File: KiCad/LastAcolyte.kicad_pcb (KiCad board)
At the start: 2 copper layers, 170 x 170 mm, 711 parts, among them J1 USB_B, J2 Mini-DIN-6, J3 AudioJack3, J4 DB15_Female_HighDensity, J5 Conn-01x06, J6 Conn_01x02, J7 Conn_02x20_Odd_Even, Q1 PN2222A, Q2 PN2222A, Q3 PN2222A, SW1 SW_SPDT, SW2 SW_Push, U1 W65C02SxP, U10 74HC273, U11 74HC166, U12 74HC166, U13 74HC10, U14 74HC08, U15 74HC00, U16 74HC02, U17 MCP130-xxxDxTO, U18 25LCxxx, U2 AS6C4008-55PCN, U3 SST39SF040, U4 74HC161, U5 74HC590, U6 74HC590, U7 74HC590, U8 74HC245, U9 74HC377, X1 CXO_DIP8/14

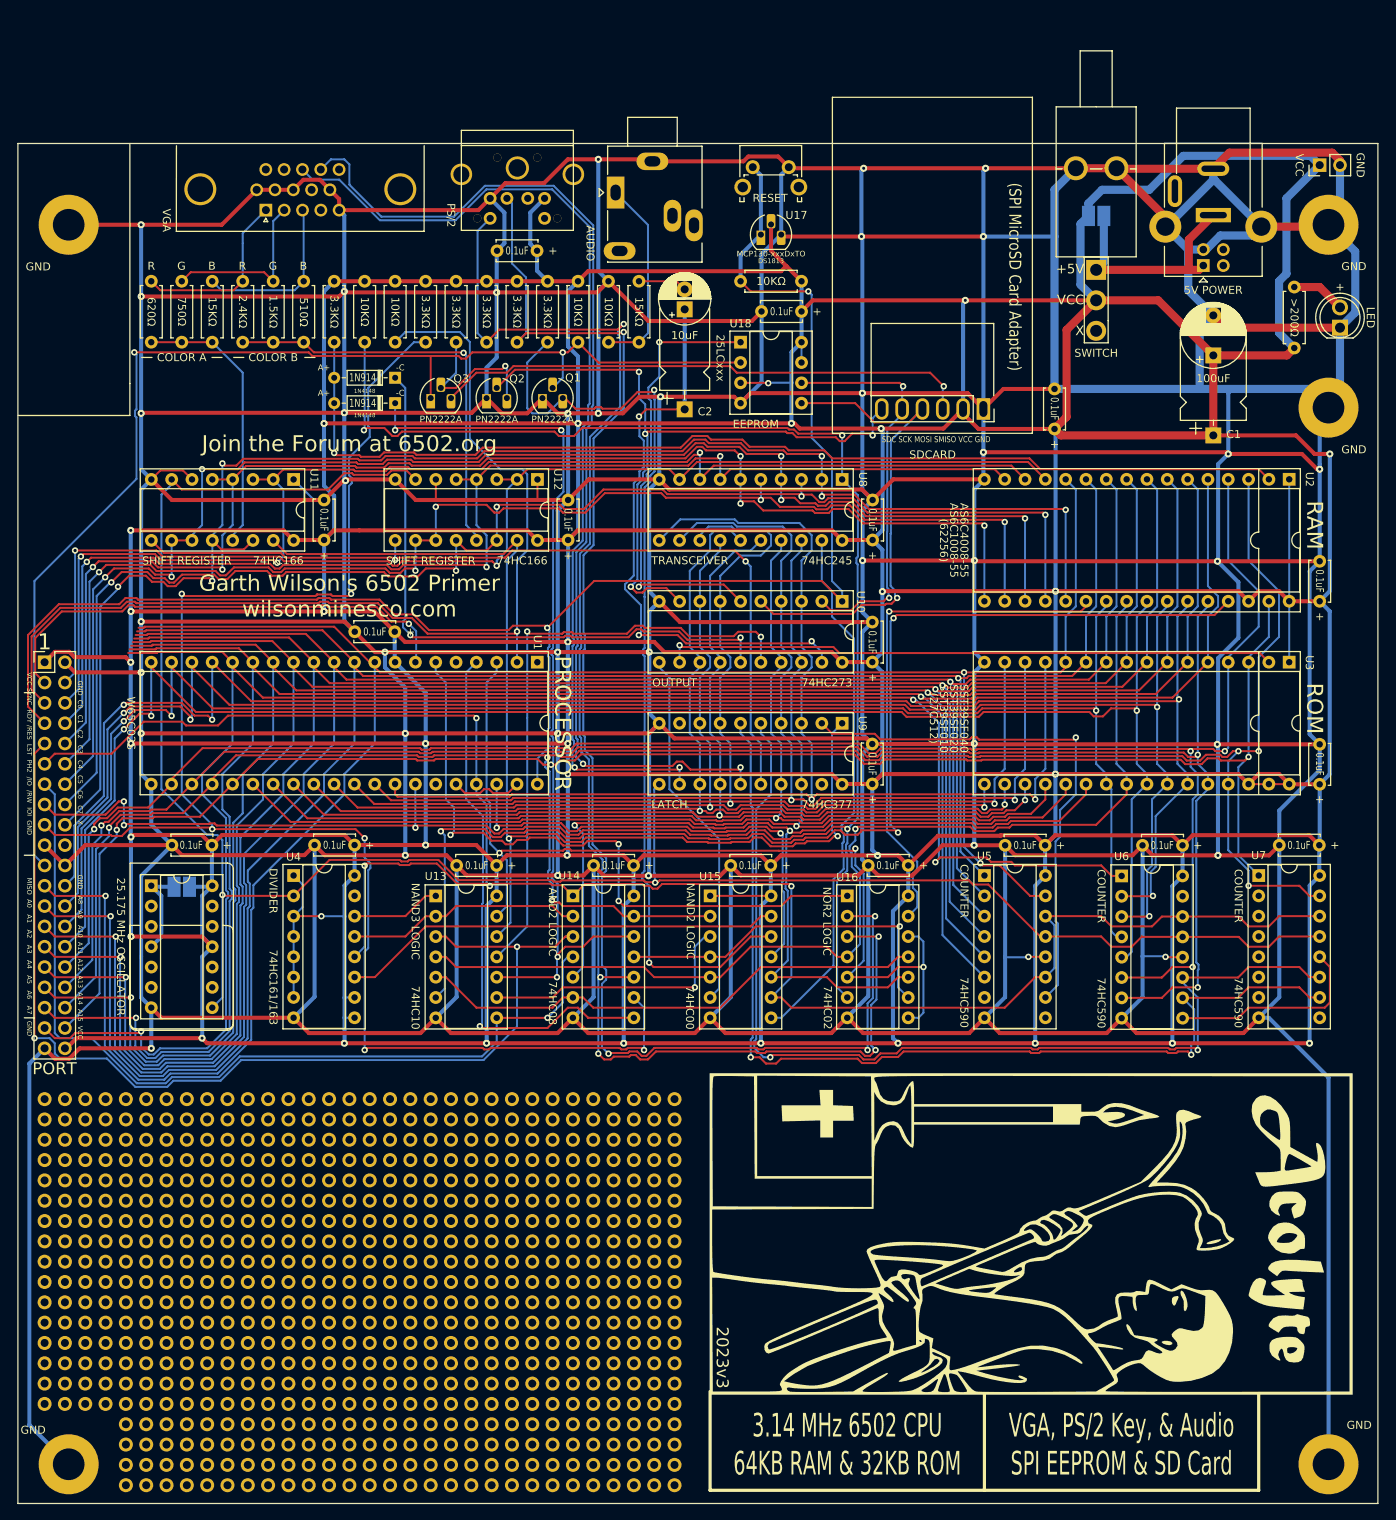
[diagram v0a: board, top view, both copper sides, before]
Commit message: Add files via upload
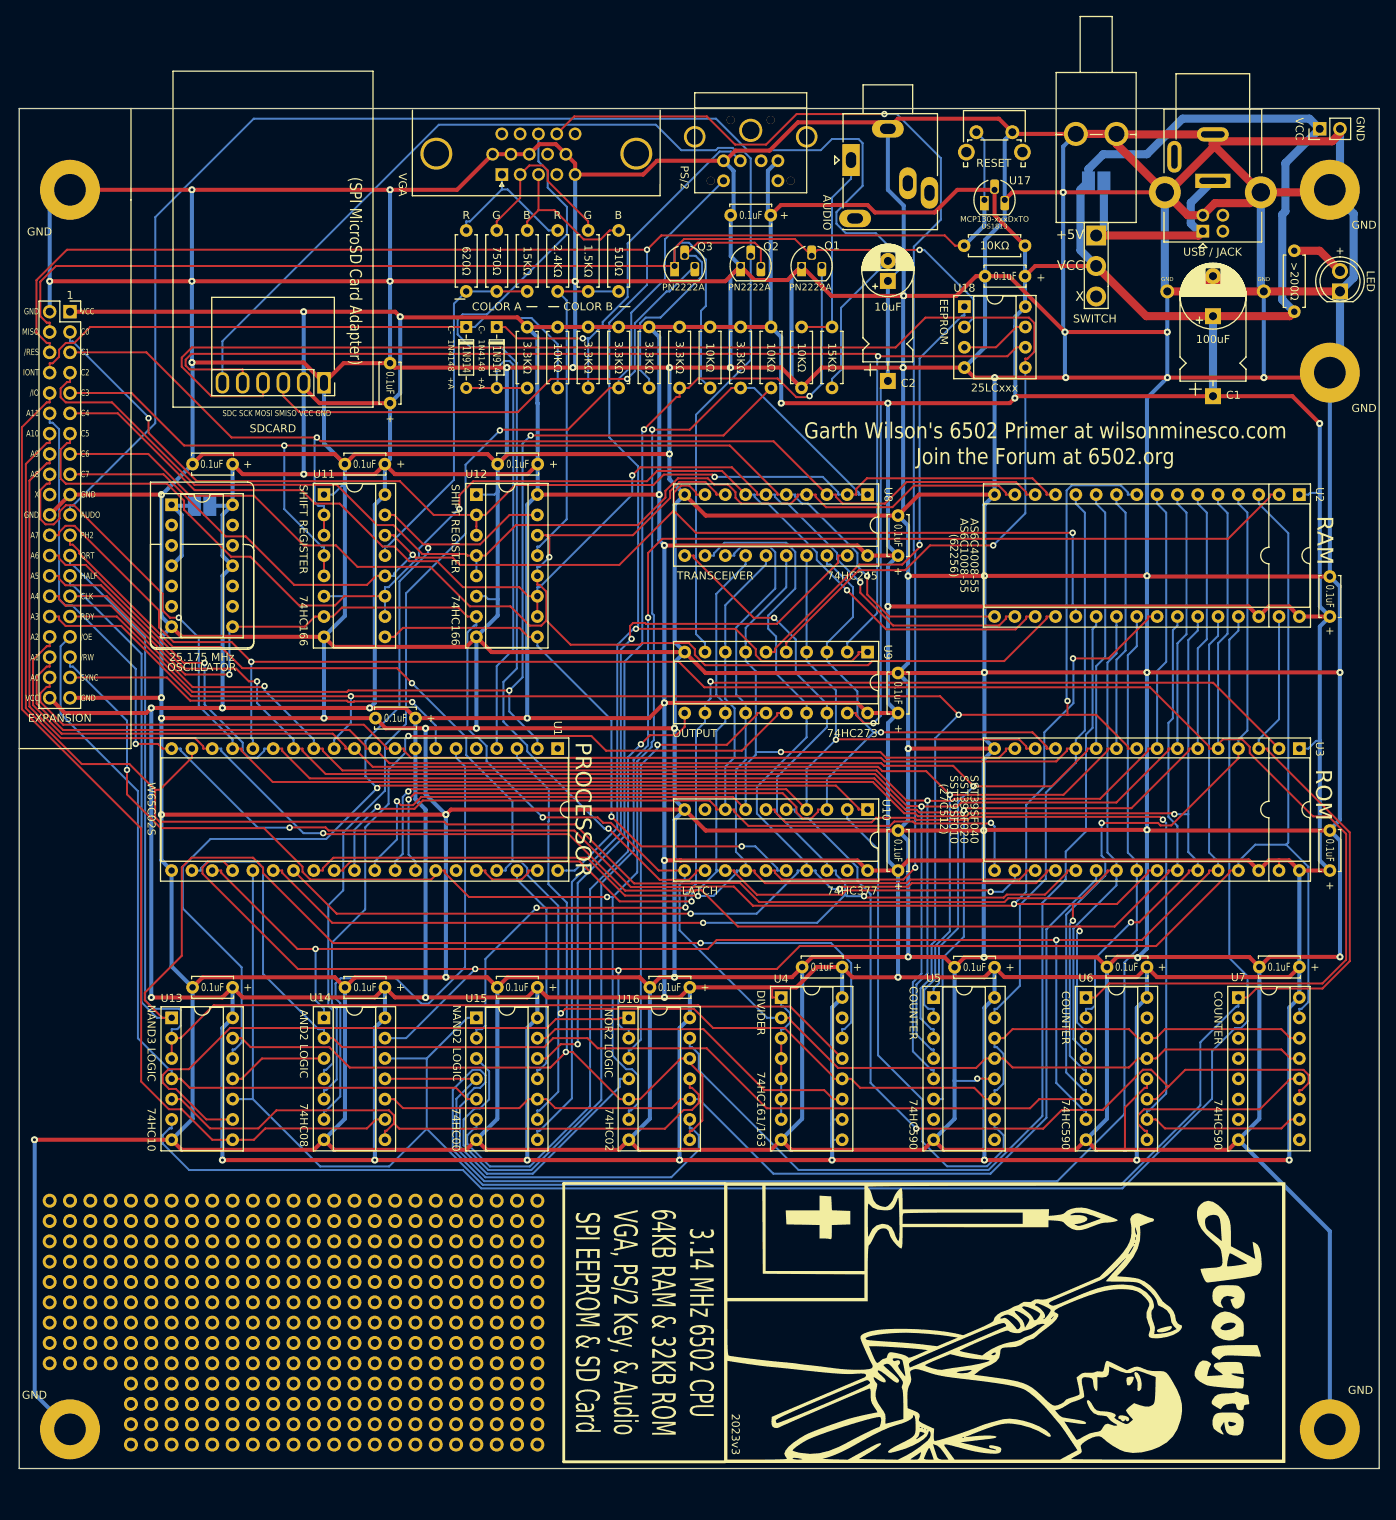
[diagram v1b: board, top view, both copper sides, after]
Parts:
- removed G100: LOGO, Library:Acolyte
- removed G200: LOGO, Library:GirlBW
- removed R15: R_US, Resistor_THT:R_Axial_DIN0207_L6.3mm_D2.5mm_P7.62mm_Horizontal
- removed the REF** at (40.0, 183.5)
- removed the REF** at (75.6, 155.6)
- removed the REF** at (101.0, 186.1)
- removed the REF** at (55.2, 181.0)
- removed the REF** at (40.0, 170.8)
- removed the REF** at (80.6, 160.7)
- removed the REF** at (29.8, 155.6)
- removed the REF** at (24.8, 170.8)
- removed the REF** at (34.9, 186.1)
- removed the REF** at (60.3, 178.4)
- removed the REF** at (98.4, 170.8)
- removed the REF** at (98.4, 145.4)
- removed the REF** at (85.7, 153.0)
- removed the REF** at (88.3, 186.1)
- removed the REF** at (50.2, 181.0)
- removed the REF** at (90.8, 188.6)
- removed the REF** at (83.2, 175.9)
- removed the REF** at (60.3, 183.5)
- removed the REF** at (75.6, 148.0)
- removed the REF** at (40.0, 173.4)
- removed the REF** at (101.0, 178.4)
- removed the REF** at (70.5, 165.7)
- removed the REF** at (60.3, 160.7)
- removed the REF** at (62.9, 165.7)
- removed the REF** at (85.7, 175.9)
- removed the REF** at (95.9, 170.8)
- removed the REF** at (27.3, 181.0)
- removed the REF** at (55.2, 165.7)
- removed the REF** at (75.6, 145.4)
- removed the REF** at (67.9, 160.7)
- removed the REF** at (50.2, 145.4)
- removed the REF** at (32.4, 186.1)
- removed the REF** at (101.0, 183.5)
- removed the REF** at (29.8, 170.8)
- removed the REF** at (95.9, 186.1)
- removed the REF** at (47.6, 158.1)
- removed the REF** at (52.7, 153.0)
- removed the REF** at (50.2, 163.2)
- removed the REF** at (67.9, 178.4)
- removed the REF** at (70.5, 150.5)
- removed the REF** at (57.8, 181.0)
- removed the REF** at (34.9, 145.4)
- removed the REF** at (29.8, 178.4)
- removed the REF** at (40.0, 160.7)
- removed the REF** at (101.0, 160.7)
- removed the REF** at (34.9, 173.4)
- removed the REF** at (42.5, 191.1)
- removed the REF** at (50.2, 193.7)
- removed the REF** at (65.4, 150.5)
- removed the REF** at (22.2, 150.5)
- removed the REF** at (73.0, 191.1)
- removed the REF** at (45.1, 188.6)
- removed the REF** at (101.0, 163.2)
- removed the REF** at (34.9, 160.7)
- removed the REF** at (60.3, 188.6)
- removed the REF** at (42.5, 165.7)
- removed the REF** at (22.2, 170.8)
- removed the REF** at (67.9, 150.5)
- removed the REF** at (27.3, 155.6)
- removed the REF** at (98.4, 193.7)
- removed the REF** at (62.9, 153.0)
- removed the REF** at (57.8, 186.1)
- removed the REF** at (80.6, 153.0)
- removed the REF** at (24.8, 175.9)
- removed the REF** at (70.5, 145.4)
- removed the REF** at (90.8, 160.7)
- removed the REF** at (73.0, 148.0)
- removed the REF** at (85.7, 155.6)
- removed the REF** at (57.8, 160.7)
- removed the REF** at (55.2, 186.1)
- removed the REF** at (52.7, 170.8)
- removed the REF** at (45.1, 155.6)
- removed the REF** at (57.8, 188.6)
- removed the REF** at (95.9, 148.0)
- removed the REF** at (32.4, 148.0)
- removed the REF** at (22.2, 183.5)
- removed the REF** at (65.4, 165.7)
- removed the REF** at (52.7, 150.5)
- removed the REF** at (34.9, 163.2)
- removed the REF** at (75.6, 178.4)
- removed the REF** at (50.2, 188.6)
- removed the REF** at (27.3, 173.4)
- removed the REF** at (101.0, 155.6)
- removed the REF** at (78.1, 168.3)
- removed the REF** at (95.9, 175.9)
- removed the REF** at (29.8, 173.4)
- removed the REF** at (45.1, 193.7)
- removed the REF** at (78.1, 183.5)
- removed the REF** at (27.3, 153.0)
- removed the REF** at (93.3, 160.7)
- removed the REF** at (70.5, 158.1)
- removed the REF** at (47.6, 155.6)
- removed the REF** at (73.0, 175.9)
- removed the REF** at (98.4, 173.4)
- removed the REF** at (37.5, 170.8)
- removed the REF** at (88.3, 193.7)
- removed the REF** at (62.9, 181.0)
- removed the REF** at (65.4, 163.2)
- removed the REF** at (75.6, 165.7)
- removed the REF** at (98.4, 175.9)
- removed the REF** at (50.2, 158.1)
- removed the REF** at (83.2, 188.6)
- removed the REF** at (88.3, 158.1)
- removed the REF** at (65.4, 148.0)
- removed the REF** at (85.7, 150.5)
- removed the REF** at (29.8, 150.5)
- removed the REF** at (47.6, 175.9)
- removed the REF** at (34.9, 175.9)
- removed the REF** at (85.7, 168.3)
- removed the REF** at (57.8, 170.8)
- removed the REF** at (47.6, 165.7)
- removed the REF** at (62.9, 148.0)
- removed the REF** at (42.5, 145.4)
- removed the REF** at (45.1, 191.1)
- removed the REF** at (75.6, 163.2)
- removed the REF** at (95.9, 145.4)
- removed the REF** at (32.4, 155.6)
- removed the REF** at (47.6, 168.3)
- removed the REF** at (65.4, 153.0)
- removed the REF** at (32.4, 150.5)
- removed the REF** at (60.3, 150.5)
- removed the REF** at (47.6, 148.0)
- removed the REF** at (88.3, 165.7)
- removed the REF** at (70.5, 181.0)
- removed the REF** at (42.5, 186.1)
- removed the REF** at (73.0, 173.4)
- removed the REF** at (67.9, 191.1)
- removed the REF** at (78.1, 163.2)
- removed the REF** at (57.8, 175.9)
- removed the REF** at (65.4, 191.1)
- removed the REF** at (27.3, 158.1)
- removed the REF** at (34.9, 170.8)
- removed the REF** at (55.2, 158.1)
- removed the REF** at (90.8, 181.0)
- removed the REF** at (78.1, 170.8)
- removed the REF** at (90.8, 153.0)
- removed the REF** at (83.2, 160.7)
- removed the REF** at (93.3, 150.5)
- removed the REF** at (80.6, 165.7)
- removed the REF** at (47.6, 183.5)
- removed the REF** at (73.0, 178.4)
- removed the REF** at (85.7, 191.1)
- removed the REF** at (88.3, 175.9)
- removed the REF** at (67.9, 183.5)
- removed the REF** at (60.3, 155.6)
- removed the REF** at (57.8, 178.4)
- removed the REF** at (50.2, 160.7)
- removed the REF** at (67.9, 170.8)
- removed the REF** at (85.7, 188.6)
- removed the REF** at (37.5, 186.1)
- removed the REF** at (55.2, 153.0)
- removed the REF** at (37.5, 178.4)
- removed the REF** at (78.1, 153.0)
- removed the REF** at (24.8, 155.6)
- removed the REF** at (50.2, 170.8)
- removed the REF** at (22.2, 155.6)
- removed the REF** at (90.8, 165.7)
- removed the REF** at (65.4, 173.4)
- removed the REF** at (93.3, 188.6)
- removed the REF** at (32.4, 165.7)
- removed the REF** at (83.2, 148.0)
- removed the REF** at (37.5, 153.0)
- removed the REF** at (95.9, 178.4)
- removed the REF** at (93.3, 191.1)
- removed the REF** at (90.8, 175.9)
- removed the REF** at (75.6, 186.1)
- removed the REF** at (55.2, 170.8)
- removed the REF** at (32.4, 173.4)
- removed the REF** at (42.5, 158.1)
- removed the REF** at (83.2, 193.7)
- removed the REF** at (83.2, 158.1)
- removed the REF** at (55.2, 145.4)
- removed the REF** at (34.9, 155.6)
- removed the REF** at (32.4, 160.7)
- removed the REF** at (24.8, 145.4)
- removed the REF** at (101.0, 153.0)
- removed the REF** at (83.2, 186.1)
- removed the REF** at (32.4, 158.1)
- removed the REF** at (93.3, 155.6)
- removed the REF** at (83.2, 170.8)
- removed the REF** at (90.8, 193.7)
- removed the REF** at (88.3, 148.0)
- removed the REF** at (22.2, 153.0)
- removed the REF** at (45.1, 168.3)
- removed the REF** at (95.9, 168.3)
- removed the REF** at (83.2, 145.4)
- removed the REF** at (95.9, 153.0)
- removed the REF** at (98.4, 178.4)
- removed the REF** at (93.3, 145.4)
- removed the REF** at (78.1, 193.7)
- removed the REF** at (40.0, 188.6)
- removed the REF** at (45.1, 148.0)
- removed the REF** at (47.6, 181.0)
- removed the REF** at (78.1, 148.0)
- removed the REF** at (50.2, 155.6)
- removed the REF** at (50.2, 178.4)
- removed the REF** at (101.0, 173.4)
- removed the REF** at (60.3, 153.0)
- removed the REF** at (62.9, 168.3)
- removed the REF** at (85.7, 148.0)
- removed the REF** at (60.3, 165.7)
- removed the REF** at (40.0, 150.5)
- removed the REF** at (50.2, 186.1)
- removed the REF** at (85.7, 165.7)
- removed the REF** at (27.3, 183.5)
- removed the REF** at (85.7, 186.1)
- removed the REF** at (37.5, 155.6)
- removed the REF** at (32.4, 145.4)
- removed the REF** at (65.4, 168.3)
- removed the REF** at (47.6, 163.2)
- removed the REF** at (80.6, 178.4)
- removed the REF** at (93.3, 153.0)
- removed the REF** at (93.3, 193.7)
- removed the REF** at (52.7, 191.1)
- removed the REF** at (73.0, 165.7)
- removed the REF** at (93.3, 173.4)
- removed the REF** at (70.5, 153.0)
- removed the REF** at (50.2, 183.5)
- removed the REF** at (62.9, 173.4)
- removed the REF** at (95.9, 163.2)
- removed the REF** at (47.6, 145.4)
- removed the REF** at (75.6, 173.4)
- removed the REF** at (67.9, 173.4)
- removed the REF** at (57.8, 158.1)
- removed the REF** at (27.3, 165.7)
- removed the REF** at (34.9, 153.0)
- removed the REF** at (32.4, 175.9)
- removed the REF** at (80.6, 148.0)
- removed the REF** at (40.0, 186.1)
- removed the REF** at (98.4, 153.0)
- removed the REF** at (67.9, 186.1)
- removed the REF** at (85.7, 145.4)
- removed the REF** at (57.8, 150.5)
- removed the REF** at (24.8, 183.5)
- removed the REF** at (98.4, 163.2)
- removed the REF** at (67.9, 163.2)
- removed the REF** at (95.9, 160.7)
- removed the REF** at (22.2, 160.7)
- removed the REF** at (22.2, 181.0)
- removed the REF** at (62.9, 188.6)
- removed the REF** at (88.3, 178.4)
- removed the REF** at (29.8, 165.7)
- removed the REF** at (75.6, 183.5)
- removed the REF** at (37.5, 173.4)
- removed the REF** at (62.9, 183.5)
- removed the REF** at (73.0, 188.6)
- removed the REF** at (24.8, 173.4)
- removed the REF** at (29.8, 183.5)
- removed the REF** at (80.6, 175.9)
- removed the REF** at (32.4, 168.3)
- removed the REF** at (27.3, 160.7)
- removed the REF** at (85.7, 160.7)
- removed the REF** at (32.4, 153.0)
- removed the REF** at (80.6, 168.3)
- removed the REF** at (80.6, 186.1)
- removed the REF** at (60.3, 168.3)
- removed the REF** at (55.2, 168.3)
- removed the REF** at (37.5, 158.1)
- removed the REF** at (90.8, 148.0)
- removed the REF** at (47.6, 178.4)
- removed the REF** at (85.7, 163.2)
- removed the REF** at (78.1, 191.1)
- removed the REF** at (98.4, 183.5)
- removed the REF** at (32.4, 181.0)
- removed the REF** at (65.4, 193.7)
- removed the REF** at (37.5, 168.3)
- removed the REF** at (60.3, 158.1)
- removed the REF** at (45.1, 145.4)
- removed the REF** at (24.8, 158.1)
- removed the REF** at (85.7, 158.1)
- removed the REF** at (65.4, 188.6)
- removed the REF** at (47.6, 153.0)
- removed the REF** at (93.3, 163.2)
- removed the REF** at (65.4, 155.6)
- removed the REF** at (50.2, 165.7)
- removed the REF** at (83.2, 150.5)
- removed the REF** at (42.5, 178.4)
- removed the REF** at (57.8, 168.3)
- removed the REF** at (60.3, 191.1)
- removed the REF** at (22.2, 165.7)
- removed the REF** at (73.0, 160.7)
- removed the REF** at (62.9, 155.6)
- removed the REF** at (57.8, 183.5)
- removed the REF** at (93.3, 170.8)
- removed the REF** at (37.5, 145.4)
- removed the REF** at (47.6, 188.6)
- removed the REF** at (73.0, 153.0)
- removed the REF** at (88.3, 183.5)
- removed the REF** at (70.5, 186.1)
- removed the REF** at (29.8, 181.0)
- removed the REF** at (42.5, 155.6)
- removed the REF** at (90.8, 145.4)
- removed the REF** at (22.2, 178.4)
- removed the REF** at (42.5, 153.0)
- removed the REF** at (85.7, 170.8)
- removed the REF** at (75.6, 181.0)
- removed the REF** at (32.4, 188.6)
- removed the REF** at (98.4, 168.3)
- removed the REF** at (73.0, 181.0)
- removed the REF** at (65.4, 186.1)
- removed the REF** at (80.6, 158.1)
- removed the REF** at (101.0, 175.9)
- removed the REF** at (101.0, 181.0)
- removed the REF** at (83.2, 183.5)
- removed the REF** at (34.9, 183.5)
- removed the REF** at (50.2, 168.3)
- removed the REF** at (98.4, 186.1)
- removed the REF** at (57.8, 173.4)
- removed the REF** at (45.1, 181.0)
- removed the REF** at (47.6, 170.8)
- removed the REF** at (75.6, 191.1)
- removed the REF** at (78.1, 178.4)
- removed the REF** at (27.3, 168.3)
- removed the REF** at (98.4, 160.7)
- removed the REF** at (83.2, 181.0)
- removed the REF** at (34.9, 181.0)
- removed the REF** at (75.6, 160.7)
- removed the REF** at (88.3, 168.3)
- removed the REF** at (40.0, 181.0)
- removed the REF** at (62.9, 163.2)
- removed the REF** at (75.6, 175.9)
- removed the REF** at (50.2, 148.0)
- removed the REF** at (45.1, 173.4)
- removed the REF** at (98.4, 148.0)
- removed the REF** at (75.6, 168.3)
- removed the REF** at (37.5, 193.7)
- removed the REF** at (40.0, 175.9)
- removed the REF** at (75.6, 170.8)
- removed the REF** at (55.2, 163.2)
- removed the REF** at (90.8, 163.2)
- removed the REF** at (52.7, 148.0)
- removed the REF** at (47.6, 150.5)
- removed the REF** at (40.0, 193.7)
- removed the REF** at (27.3, 170.8)
- removed the REF** at (27.3, 178.4)
- removed the REF** at (37.5, 160.7)
- removed the REF** at (40.0, 168.3)
- removed the REF** at (70.5, 160.7)
- removed the REF** at (70.5, 183.5)
- removed the REF** at (29.8, 158.1)
- removed the REF** at (22.2, 175.9)
- removed the REF** at (29.8, 160.7)
- removed the REF** at (101.0, 165.7)
- removed the REF** at (22.2, 163.2)
- removed the REF** at (22.2, 148.0)
- removed the REF** at (98.4, 158.1)
- removed the REF** at (60.3, 186.1)
- removed the REF** at (85.7, 181.0)
- removed the REF** at (62.9, 186.1)
- removed the REF** at (67.9, 181.0)
- removed the REF** at (65.4, 181.0)
- removed the REF** at (40.0, 191.1)
- removed the REF** at (101.0, 150.5)
- removed the REF** at (93.3, 186.1)
- removed the REF** at (47.6, 160.7)
- removed the REF** at (65.4, 170.8)
- removed the REF** at (101.0, 188.6)
- removed the REF** at (60.3, 170.8)
- removed the REF** at (32.4, 191.1)
- removed the REF** at (47.6, 186.1)
- removed the REF** at (34.9, 150.5)
- removed the REF** at (42.5, 148.0)
- removed the REF** at (45.1, 150.5)
- removed the REF** at (55.2, 148.0)
- removed the REF** at (75.6, 188.6)
- removed the REF** at (101.0, 148.0)
- removed the REF** at (65.4, 175.9)
- removed the REF** at (55.2, 160.7)
- removed the REF** at (93.3, 178.4)
- removed the REF** at (78.1, 150.5)
- removed the REF** at (52.7, 186.1)
- removed the REF** at (40.0, 158.1)
- removed the REF** at (83.2, 163.2)
- removed the REF** at (52.7, 168.3)
- removed the REF** at (101.0, 191.1)
- removed the REF** at (27.3, 145.4)
- removed the REF** at (73.0, 186.1)
- removed the REF** at (78.1, 165.7)
- removed the REF** at (57.8, 191.1)
- removed the REF** at (95.9, 183.5)
- removed the REF** at (90.8, 173.4)
- removed the REF** at (101.0, 170.8)
- removed the REF** at (73.0, 155.6)
- removed the REF** at (90.8, 150.5)
- removed the REF** at (50.2, 175.9)
- removed the REF** at (24.8, 168.3)
- removed the REF** at (29.8, 168.3)
- removed the REF** at (57.8, 193.7)
- removed the REF** at (67.9, 153.0)
- removed the REF** at (34.9, 178.4)
- removed the REF** at (32.4, 170.8)
- removed the REF** at (78.1, 188.6)
- removed the REF** at (95.9, 165.7)
- removed the REF** at (93.3, 165.7)
- removed the REF** at (42.5, 163.2)
- removed the REF** at (29.8, 145.4)
- removed the REF** at (40.0, 155.6)
- removed the REF** at (55.2, 175.9)
- removed the REF** at (98.4, 188.6)
- removed the REF** at (65.4, 183.5)
- removed the REF** at (75.6, 158.1)
- removed the REF** at (101.0, 168.3)
- removed the REF** at (45.1, 163.2)
- removed the REF** at (88.3, 181.0)
- removed the REF** at (88.3, 188.6)
- removed the REF** at (95.9, 193.7)
- removed the REF** at (52.7, 181.0)
- removed the REF** at (34.9, 193.7)
- removed the REF** at (24.8, 178.4)
- removed the REF** at (34.9, 168.3)
- removed the REF** at (42.5, 168.3)
- removed the REF** at (83.2, 168.3)
- removed the REF** at (90.8, 186.1)
- removed the REF** at (22.2, 145.4)
- removed the REF** at (60.3, 181.0)
- removed the REF** at (70.5, 173.4)
- removed the REF** at (78.1, 145.4)
- removed the REF** at (62.9, 193.7)
- removed the REF** at (78.1, 186.1)
- removed the REF** at (80.6, 173.4)
- removed the REF** at (88.3, 191.1)
- removed the REF** at (32.4, 163.2)
- removed the REF** at (42.5, 175.9)
- removed the REF** at (80.6, 163.2)
- removed the REF** at (70.5, 193.7)
- removed the REF** at (37.5, 150.5)
- removed the REF** at (83.2, 155.6)
- removed the REF** at (52.7, 193.7)
- removed the REF** at (45.1, 170.8)
- removed the REF** at (78.1, 158.1)
- removed the REF** at (45.1, 178.4)
- removed the REF** at (29.8, 153.0)
- removed the REF** at (83.2, 165.7)
- removed the REF** at (42.5, 173.4)
- removed the REF** at (65.4, 160.7)
- removed the REF** at (45.1, 160.7)
- removed the REF** at (42.5, 150.5)
- removed the REF** at (42.5, 183.5)
- removed the REF** at (55.2, 155.6)
- removed the REF** at (40.0, 163.2)
- removed the REF** at (62.9, 160.7)
- removed the REF** at (80.6, 145.4)
- removed the REF** at (85.7, 183.5)
- removed the REF** at (70.5, 155.6)
- removed the REF** at (88.3, 160.7)
- removed the REF** at (62.9, 145.4)
- removed the REF** at (95.9, 150.5)
- removed the REF** at (62.9, 178.4)
- removed the REF** at (22.2, 173.4)
- removed the REF** at (52.7, 145.4)
- removed the REF** at (24.8, 150.5)
- removed the REF** at (40.0, 145.4)
- removed the REF** at (70.5, 188.6)
- removed the REF** at (70.5, 191.1)
- removed the REF** at (47.6, 193.7)
- removed the REF** at (45.1, 183.5)
- removed the REF** at (67.9, 188.6)
- removed the REF** at (85.7, 193.7)
- removed the REF** at (60.3, 148.0)
- removed the REF** at (52.7, 183.5)
- removed the REF** at (60.3, 163.2)
- removed the REF** at (34.9, 191.1)
- removed the REF** at (62.9, 150.5)
- removed the REF** at (85.7, 173.4)
- removed the REF** at (32.4, 183.5)
- removed the REF** at (47.6, 191.1)
- removed the REF** at (60.3, 175.9)
- removed the REF** at (80.6, 193.7)
- removed the REF** at (32.4, 178.4)
- removed the REF** at (45.1, 158.1)
- removed the REF** at (95.9, 181.0)
- removed the REF** at (65.4, 178.4)
- removed the REF** at (29.8, 175.9)
- removed the REF** at (73.0, 145.4)
- removed the REF** at (40.0, 165.7)
- removed the REF** at (40.0, 153.0)
- removed the REF** at (73.0, 158.1)
- removed the REF** at (55.2, 178.4)
- removed the REF** at (57.8, 165.7)
- removed the REF** at (32.4, 193.7)
- removed the REF** at (67.9, 148.0)
- removed the REF** at (55.2, 191.1)
- removed the REF** at (24.8, 160.7)
- removed the REF** at (88.3, 163.2)
- removed the REF** at (75.6, 150.5)
- removed the REF** at (90.8, 191.1)
- removed the REF** at (52.7, 165.7)
- removed the REF** at (73.0, 170.8)
- removed the REF** at (34.9, 158.1)
- removed the REF** at (88.3, 150.5)
- removed the REF** at (70.5, 178.4)
- removed the REF** at (22.2, 168.3)
- removed the REF** at (83.2, 153.0)
- removed the REF** at (62.9, 175.9)
- removed the REF** at (88.3, 155.6)
- removed the REF** at (37.5, 191.1)
- removed the REF** at (95.9, 173.4)
- removed the REF** at (83.2, 191.1)
- removed the REF** at (57.8, 163.2)
- removed the REF** at (27.3, 148.0)
- removed the REF** at (95.9, 191.1)
- removed the REF** at (95.9, 155.6)
- removed the REF** at (60.3, 145.4)
- removed the REF** at (52.7, 155.6)
- removed the REF** at (22.2, 158.1)
- removed the REF** at (37.5, 181.0)
- removed the REF** at (90.8, 178.4)
- removed the REF** at (50.2, 191.1)
- removed the REF** at (85.7, 178.4)
- removed the REF** at (67.9, 155.6)
- removed the REF** at (75.6, 193.7)
- removed the REF** at (95.9, 158.1)
- removed the REF** at (34.9, 148.0)
- removed the REF** at (42.5, 188.6)
- removed the REF** at (45.1, 165.7)
- removed the REF** at (93.3, 183.5)
- removed the REF** at (37.5, 148.0)
- removed the REF** at (78.1, 155.6)
- removed the REF** at (42.5, 160.7)
- removed the REF** at (98.4, 150.5)
- removed the REF** at (60.3, 173.4)
- removed the REF** at (67.9, 165.7)
- removed the REF** at (98.4, 191.1)
- removed the REF** at (88.3, 153.0)
- removed the REF** at (93.3, 158.1)
- removed the REF** at (37.5, 175.9)
- removed the REF** at (101.0, 145.4)
- removed the REF** at (93.3, 168.3)
- removed the REF** at (29.8, 148.0)
- removed the REF** at (55.2, 173.4)
- removed the REF** at (42.5, 181.0)
- removed the REF** at (83.2, 178.4)
- removed the REF** at (73.0, 163.2)
- removed the REF** at (98.4, 181.0)
- removed the REF** at (83.2, 173.4)
- removed the REF** at (80.6, 170.8)
- removed the REF** at (70.5, 175.9)
- removed the REF** at (70.5, 168.3)
- removed the REF** at (52.7, 175.9)
- removed the REF** at (67.9, 168.3)
- removed the REF** at (88.3, 145.4)
- removed the REF** at (80.6, 181.0)
- removed the REF** at (50.2, 173.4)
- removed the REF** at (90.8, 183.5)
- removed the REF** at (98.4, 165.7)
- removed the REF** at (78.1, 175.9)
- removed the REF** at (80.6, 188.6)
- removed the REF** at (52.7, 173.4)
- removed the REF** at (40.0, 148.0)
- removed the REF** at (52.7, 188.6)
- removed the REF** at (37.5, 163.2)
- removed the REF** at (45.1, 186.1)
- removed the REF** at (80.6, 183.5)
- removed the REF** at (101.0, 158.1)
- removed the REF** at (50.2, 153.0)
- removed the REF** at (37.5, 165.7)
- removed the REF** at (55.2, 183.5)
- removed the REF** at (90.8, 155.6)
- removed the REF** at (57.8, 148.0)
- removed the REF** at (24.8, 153.0)
- removed the REF** at (62.9, 170.8)
- removed the REF** at (62.9, 191.1)
- removed the REF** at (57.8, 153.0)
- removed the REF** at (40.0, 178.4)
- removed the REF** at (24.8, 148.0)
- removed the REF** at (67.9, 175.9)
- removed the REF** at (45.1, 153.0)
- removed the REF** at (75.6, 153.0)
- removed the REF** at (37.5, 183.5)
- removed the REF** at (90.8, 168.3)
- removed the REF** at (88.3, 170.8)
- removed the REF** at (90.8, 170.8)
- removed the REF** at (67.9, 158.1)
- removed the REF** at (42.5, 170.8)
- removed the REF** at (73.0, 193.7)
- removed the REF** at (90.8, 158.1)
- removed the REF** at (73.0, 183.5)
- removed the REF** at (93.3, 181.0)
- removed the REF** at (65.4, 158.1)
- removed the REF** at (78.1, 160.7)
- removed the REF** at (93.3, 175.9)
- removed the REF** at (52.7, 163.2)
- removed the REF** at (95.9, 188.6)
- removed the REF** at (50.2, 150.5)
- removed the REF** at (55.2, 188.6)
- removed the REF** at (55.2, 150.5)
- removed the REF** at (24.8, 165.7)
- removed the REF** at (78.1, 173.4)
- removed the REF** at (34.9, 165.7)
- removed the REF** at (67.9, 193.7)
- removed the REF** at (57.8, 155.6)
- removed the REF** at (80.6, 155.6)
- removed the REF** at (45.1, 175.9)
- removed the REF** at (98.4, 155.6)
- removed the REF** at (52.7, 160.7)
- removed the REF** at (101.0, 193.7)
- removed the REF** at (42.5, 193.7)
- removed the REF** at (93.3, 148.0)
- removed the REF** at (27.3, 163.2)
- removed the REF** at (65.4, 145.4)
- removed the REF** at (70.5, 170.8)
- removed the REF** at (70.5, 148.0)
- removed the REF** at (88.3, 173.4)
- removed the REF** at (27.3, 150.5)
- removed the REF** at (24.8, 181.0)
- removed the REF** at (70.5, 163.2)
- removed the REF** at (52.7, 158.1)
- removed the REF** at (37.5, 188.6)
- removed the REF** at (60.3, 193.7)
- removed the REF** at (29.8, 163.2)
- removed the REF** at (62.9, 158.1)
- removed the REF** at (78.1, 181.0)
- removed the REF** at (34.9, 188.6)
- removed the REF** at (52.7, 178.4)
- removed the REF** at (80.6, 150.5)
- removed the REF** at (73.0, 150.5)
- removed the REF** at (80.6, 191.1)
- removed the REF** at (27.3, 175.9)
- removed the REF** at (57.8, 145.4)
- removed the REF** at (24.8, 163.2)
- removed the REF** at (55.2, 193.7)
- removed the REF** at (47.6, 173.4)
- removed the REF** at (73.0, 168.3)
- removed the REF** at (67.9, 145.4)
- added G99: LOGO, Library:AcolyteLogoSmall, F.Cu at (142.2, 173.4)
- added R20: R_US, Resistor_THT:R_Axial_DIN0207_L6.3mm_D2.5mm_P7.62mm_Horizontal, F.Cu at (86.4, 56.5)
- added REF**: CustomTestPoint, Library:CustomTestPoint, F.Cu at (73.7, 186.1)
- added REF**: CustomTestPoint, Library:CustomTestPoint, F.Cu at (48.3, 181.0)
- added REF**: CustomTestPoint, Library:CustomTestPoint, F.Cu at (83.8, 158.1)
- added REF**: CustomTestPoint, Library:CustomTestPoint, F.Cu at (50.8, 168.3)
- added REF**: CustomTestPoint, Library:CustomTestPoint, F.Cu at (66.0, 168.3)
- added REF**: CustomTestPoint, Library:CustomTestPoint, F.Cu at (53.3, 173.4)
- added REF**: CustomTestPoint, Library:CustomTestPoint, F.Cu at (35.6, 175.9)
- added REF**: CustomTestPoint, Library:CustomTestPoint, F.Cu at (25.4, 170.8)
- added REF**: CustomTestPoint, Library:CustomTestPoint, F.Cu at (53.3, 160.7)
- added REF**: CustomTestPoint, Library:CustomTestPoint, F.Cu at (58.4, 173.4)
- added REF**: CustomTestPoint, Library:CustomTestPoint, F.Cu at (63.5, 186.1)
- added REF**: CustomTestPoint, Library:CustomTestPoint, F.Cu at (61.0, 178.4)
- added REF**: CustomTestPoint, Library:CustomTestPoint, F.Cu at (35.6, 173.4)
- added REF**: CustomTestPoint, Library:CustomTestPoint, F.Cu at (71.1, 168.3)
- added REF**: CustomTestPoint, Library:CustomTestPoint, F.Cu at (73.7, 168.3)
- added REF**: CustomTestPoint, Library:CustomTestPoint, F.Cu at (76.2, 160.7)
- added REF**: CustomTestPoint, Library:CustomTestPoint, F.Cu at (78.7, 163.2)
- added REF**: CustomTestPoint, Library:CustomTestPoint, F.Cu at (25.4, 160.7)
- added REF**: CustomTestPoint, Library:CustomTestPoint, F.Cu at (50.8, 186.1)
- added REF**: CustomTestPoint, Library:CustomTestPoint, F.Cu at (78.7, 168.3)
- added REF**: CustomTestPoint, Library:CustomTestPoint, F.Cu at (38.1, 188.6)
- added REF**: CustomTestPoint, Library:CustomTestPoint, F.Cu at (66.0, 181.0)
- added REF**: CustomTestPoint, Library:CustomTestPoint, F.Cu at (27.9, 160.7)
- added REF**: CustomTestPoint, Library:CustomTestPoint, F.Cu at (83.8, 173.4)
- added REF**: CustomTestPoint, Library:CustomTestPoint, F.Cu at (71.1, 183.5)
- added REF**: CustomTestPoint, Library:CustomTestPoint, F.Cu at (45.7, 183.5)
- added REF**: CustomTestPoint, Library:CustomTestPoint, F.Cu at (66.0, 188.6)
- added REF**: CustomTestPoint, Library:CustomTestPoint, F.Cu at (55.9, 165.7)
- added REF**: CustomTestPoint, Library:CustomTestPoint, F.Cu at (45.7, 165.7)
- added REF**: CustomTestPoint, Library:CustomTestPoint, F.Cu at (48.3, 188.6)
- added REF**: CustomTestPoint, Library:CustomTestPoint, F.Cu at (45.7, 158.1)
- added REF**: CustomTestPoint, Library:CustomTestPoint, F.Cu at (38.1, 173.4)
- added REF**: CustomTestPoint, Library:CustomTestPoint, F.Cu at (66.0, 183.5)
- added REF**: CustomTestPoint, Library:CustomTestPoint, F.Cu at (81.3, 188.6)
- added REF**: CustomTestPoint, Library:CustomTestPoint, F.Cu at (55.9, 173.4)
- added REF**: CustomTestPoint, Library:CustomTestPoint, F.Cu at (48.3, 178.4)
- added REF**: CustomTestPoint, Library:CustomTestPoint, F.Cu at (25.4, 165.7)
- added REF**: CustomTestPoint, Library:CustomTestPoint, F.Cu at (81.3, 158.1)
- added REF**: CustomTestPoint, Library:CustomTestPoint, F.Cu at (22.9, 165.7)
- added REF**: CustomTestPoint, Library:CustomTestPoint, F.Cu at (33.0, 186.1)
- added REF**: CustomTestPoint, Library:CustomTestPoint, F.Cu at (45.7, 186.1)
- added REF**: CustomTestPoint, Library:CustomTestPoint, F.Cu at (53.3, 165.7)
- added REF**: CustomTestPoint, Library:CustomTestPoint, F.Cu at (68.6, 188.6)
- added REF**: CustomTestPoint, Library:CustomTestPoint, F.Cu at (35.6, 168.3)
- added REF**: CustomTestPoint, Library:CustomTestPoint, F.Cu at (73.7, 181.0)
- added REF**: CustomTestPoint, Library:CustomTestPoint, F.Cu at (58.4, 186.1)
- added REF**: CustomTestPoint, Library:CustomTestPoint, F.Cu at (43.2, 163.2)
- added REF**: CustomTestPoint, Library:CustomTestPoint, F.Cu at (45.7, 170.8)
- added REF**: CustomTestPoint, Library:CustomTestPoint, F.Cu at (48.3, 165.7)
- added REF**: CustomTestPoint, Library:CustomTestPoint, F.Cu at (83.8, 186.1)
- added REF**: CustomTestPoint, Library:CustomTestPoint, F.Cu at (71.1, 173.4)
- added REF**: CustomTestPoint, Library:CustomTestPoint, F.Cu at (33.0, 173.4)
- added REF**: CustomTestPoint, Library:CustomTestPoint, F.Cu at (58.4, 170.8)
- added REF**: CustomTestPoint, Library:CustomTestPoint, F.Cu at (61.0, 163.2)
- added REF**: CustomTestPoint, Library:CustomTestPoint, F.Cu at (35.6, 183.5)
- added REF**: CustomTestPoint, Library:CustomTestPoint, F.Cu at (38.1, 160.7)
- added REF**: CustomTestPoint, Library:CustomTestPoint, F.Cu at (27.9, 170.8)
- added REF**: CustomTestPoint, Library:CustomTestPoint, F.Cu at (30.5, 158.1)
- added REF**: CustomTestPoint, Library:CustomTestPoint, F.Cu at (38.1, 158.1)
- added REF**: CustomTestPoint, Library:CustomTestPoint, F.Cu at (45.7, 163.2)
- added REF**: CustomTestPoint, Library:CustomTestPoint, F.Cu at (38.1, 181.0)
- added REF**: CustomTestPoint, Library:CustomTestPoint, F.Cu at (50.8, 160.7)
- added REF**: CustomTestPoint, Library:CustomTestPoint, F.Cu at (71.1, 175.9)
- added REF**: CustomTestPoint, Library:CustomTestPoint, F.Cu at (53.3, 188.6)
- added REF**: CustomTestPoint, Library:CustomTestPoint, F.Cu at (81.3, 173.4)
- added REF**: CustomTestPoint, Library:CustomTestPoint, F.Cu at (63.5, 160.7)
- added REF**: CustomTestPoint, Library:CustomTestPoint, F.Cu at (33.0, 163.2)
- added REF**: CustomTestPoint, Library:CustomTestPoint, F.Cu at (43.2, 183.5)
- added REF**: CustomTestPoint, Library:CustomTestPoint, F.Cu at (33.0, 181.0)
- added REF**: CustomTestPoint, Library:CustomTestPoint, F.Cu at (61.0, 186.1)
- added REF**: CustomTestPoint, Library:CustomTestPoint, F.Cu at (25.4, 168.3)
- added REF**: CustomTestPoint, Library:CustomTestPoint, F.Cu at (53.3, 178.4)
- added REF**: CustomTestPoint, Library:CustomTestPoint, F.Cu at (58.4, 165.7)
- added REF**: CustomTestPoint, Library:CustomTestPoint, F.Cu at (40.6, 173.4)
- added REF**: CustomTestPoint, Library:CustomTestPoint, F.Cu at (58.4, 178.4)
- added REF**: CustomTestPoint, Library:CustomTestPoint, F.Cu at (30.5, 165.7)
- added REF**: CustomTestPoint, Library:CustomTestPoint, F.Cu at (40.6, 178.4)
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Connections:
- net Net-(D1-Pad2) renamed LED
- D2 pad 1: A15 -> KEY-DATA
- D2 pad 2: RAMEXP -> ~{IRQ}
- D3 pad 1: BANK-RAM -> IO-INT
- D3 pad 2: RAMEXP -> ~{IRQ}
- J7 pad 10: C3 -> ~{IO}
- J7 pad 11: PHI2 -> C4
- J7 pad 12: C4 -> A11
- J7 pad 13: ~{IO} -> C5
- J7 pad 14: C5 -> A10
- J7 pad 15: ~{RW} -> C6
- J7 pad 16: C6 -> A9
- J7 pad 17: IO-INT -> C7
- J7 pad 18: C7 -> A8
- J7 pad 21: SPI-MISO -> AUDIO-OUT
- J7 pad 23: A0 -> PHI2
- J7 pad 24: A8 -> A7
- J7 pad 25: A1 -> QUARTER
- J7 pad 26: A9 -> A6
- J7 pad 27: A2 -> HALF
- J7 pad 28: A10 -> A5
- J7 pad 29: A3 -> CLK
- J7 pad 3: SYNC -> C0
- J7 pad 30: A11 -> A4
- J7 pad 31: A4 -> RDY
- J7 pad 32: A12 -> A3
- J7 pad 33: A5 -> ~{OE}
- J7 pad 34: A13 -> A2
- J7 pad 35: A6 -> ~{RW}
- J7 pad 36: A14 -> A1
- J7 pad 37: A7 -> SYNC
- J7 pad 38: A15 -> A0
- J7 pad 4: C0 -> SPI-MISO
- J7 pad 5: RDY -> C1
- J7 pad 6: C1 -> ~{RES}
- J7 pad 7: ~{RES} -> C2
- J7 pad 8: C2 -> IO-INT
- J7 pad 9: LAST -> C3
- R16 pad 1: +5V -> ~{IRQ}
- R16 pad 2: RAMEXP -> +5V
- U10 pad 1: ~{RES} -> ~{LATCH}
- U10 pad 11: ~{OUTPUT} -> CLK
- U10 pad 12: BANK-ROM -> H-SYNC
- U10 pad 15: BANK-RAM -> V-SYNC
- U10 pad 16: IO-ENABLE -> VISIBLE
- U10 pad 19: AUDIO-OUT -> V-BLANK
- U10 pad 2: SPI-CLK -> H-RESET
- U10 pad 5: SPI-MOSI -> ~{H-RESET}
- U10 pad 6: SPI-EEPROM -> V-RESET
- U10 pad 9: SPI-SDCARD -> ~{V-RESET}
- U13 pad 11: IO-ENABLE -> MID
- U13 pad 3: LAST -> QUARTER
- U14 pad 1: PHI2 -> A13
- U14 pad 10: KEY-CLK -> ~{ROM}
- U14 pad 2: QUARTER -> A12
- U14 pad 3: LAST -> MID
- U14 pad 4: ~{IO} -> KEY-CLK
- U14 pad 5: ~{ROM} -> NMI-ENABLE
- U14 pad 6: RAMADDR -> ~{NMI}
- U14 pad 8: ~{IRQ} -> RAMADDR
- U14 pad 9: IO-INT -> ~{IO}
- U15 pad 1: +5V -> A15
- U15 pad 2: A14 -> MEM-BANK
- U15 pad 3: ~{A14} -> RAMEXP
- U16 pad 1: ~{NMI} -> ~{A14}
- U16 pad 2: KEY-DATA -> A14
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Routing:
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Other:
- board text added: "$8000-$AFFF=Banked RAM $B000-$BFFF=I/O (or RAM) $C000-$FFFF=Banked ROM"
- board text added: "/A14 A14 IOE /OE /PH2 /RW GND"
- board text added: "/RW C0 C1 C2 C3 C4 C5 C6 C7 GND"
- board text added: "3.14 MHz 6502 CPU 64KB RAM & 32KB ROM VGA, PS/2 Key, & Audio SPI EEPROM & SD Card"
- board text added: "A+ 1N4148 -C"
- board text added: "A13 A12 MID KCLK NMIE /NMI GND"
- board text added: "A15 MEMB RME HGH /OE /OUT GND"
- board text added: "AUDN GND RDY /RW MISO /MISO /SDC KCLK KDAT IONT /IRQ /IRQ /IRQ"
- board text added: "AUDT AUDT VCC VCC VCC VCC VCC VCC VCC VCC VCC KDAT IONT"
- board text added: "Bit4=MEM-BANK Bit5=IO-ENABLE Bit6=NMI-ENABLE Bit7=AUDIO-OUT"
- board text added: "C- 1N4148 +A"
- board text added: "DIP-8 DIP-40 DIP-32 DIP-32 DIP-16 DIP-16 DIP-20 DIP-20 DIP-20 DIP-16 DIP-14 DIP-14 DIP-14 DIP-14 TO-92 DIP-8 TO-92 5mm Rad 15mm Ax 5mm Dsc 2.2V DO-34 1/4W 5% 1/4W 5% 1/4W 5% 1/4W 5% 1/4W 5% 1/4W 5% 1/4W 5% 1/4W 5% 1/4W 5% 61729 5749266-1 SJ1-3513 DSub 15 SPI Mod T1B4M7QES PTS645 2.54mm"
- board text added: "GND MISO /RES IONT /IO A11 A10 A9 A8 X GND A7 A6 A5 A4 A3 A2 A1 A0 VCC"
- board text added: "Garth Wilson's 6502 Primer at wilsonminesco.com Join the Forum at 6502.org"
- board text added: "HALF QRT QRT /OE RAD /WE GND"
- board text added: "Input is through 6502 interrupts: /NMI = KEY-CLK AND NMI-ENABLE /IRQ = KEY-DATA AND IO-INT /SO = SPI-MISO (CLV, NOP, then BVS)"
- board text added: "NMI must be enabled in software to use the PS/2 Keyboard. ENABLE and BYPASS are optional. USB-to-PS/2 adapters will not work. VGA-to-HDMI adapters should work."
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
